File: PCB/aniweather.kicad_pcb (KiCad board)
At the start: 2 copper layers, 55 x 75 mm, 26 parts, among them SW1 SW_DIP_x01, SW2 SW_Push, U5 TPS63001

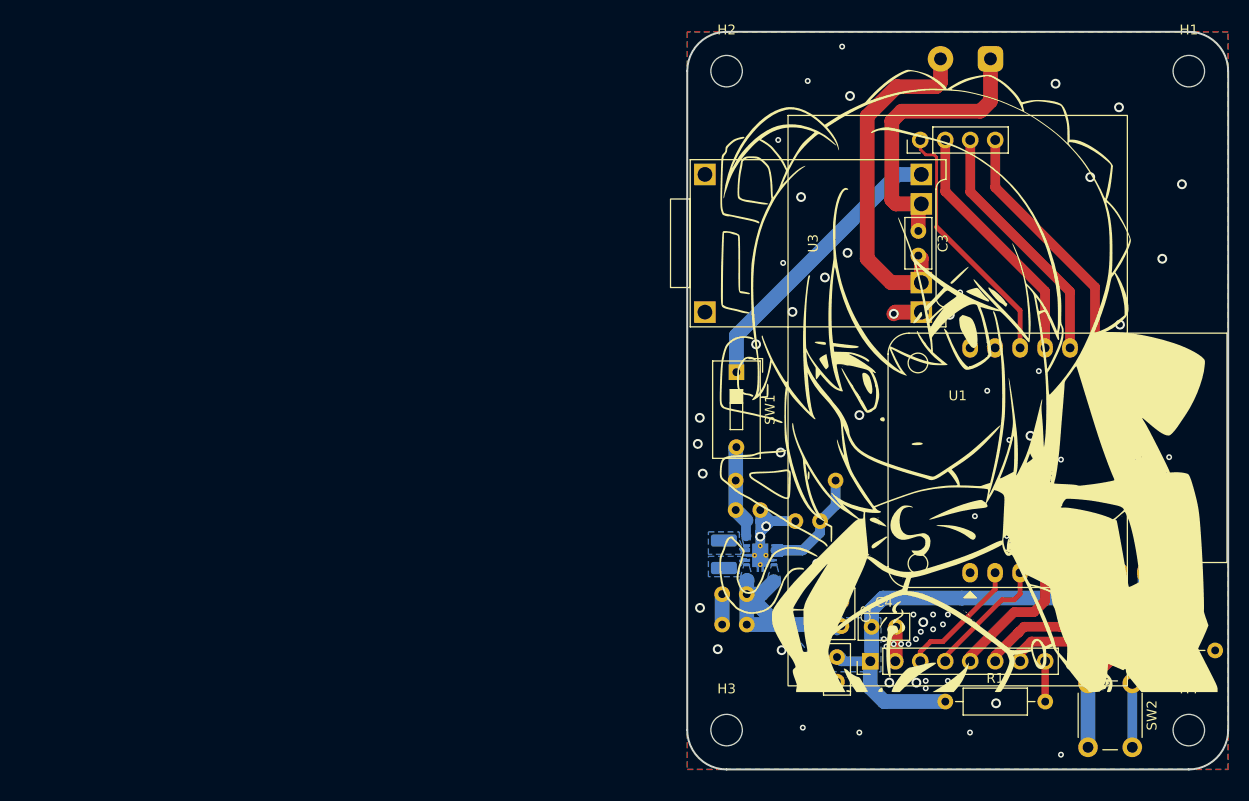
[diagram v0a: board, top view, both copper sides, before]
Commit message: Reroute board
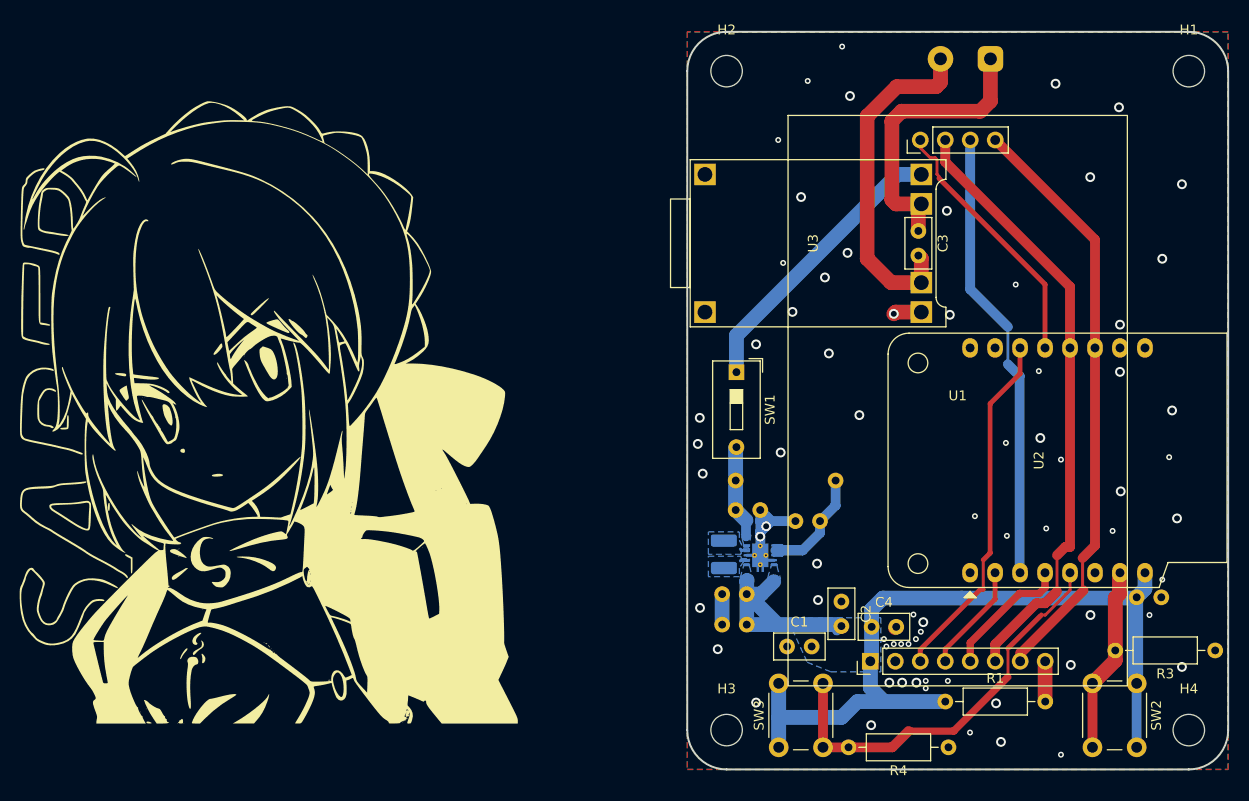
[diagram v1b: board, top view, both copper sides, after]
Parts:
- added R4: 100k, Resistor_THT:R_Axial_DIN0207_L6.3mm_D2.5mm_P10.16mm_Horizontal, F.Cu at (139.3, 136.2)
- added SW3: SW_Push, Button_Switch_THT:SW_PUSH_6mm, F.Cu at (122.0, 136.2)
- moved G1 71.2 mm to (69.2, 98.7)
- moved G2 71.2 mm to (69.2, 98.7)
- moved C1 6.21 mm to (122.8, 125.9), turned to 0 degrees
- moved SW2 0.45 mm to (158.4, 129.7)
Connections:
- U1 pad 10: SD_MISO -> MISO
- U1 pad 11: SD_SCK -> SCK
- U1 pad 5: SDA -> MOSI
- U1 pad 9: SD_MOSI -> MOSI
- U2 pad 0: SDA -> Net-(U2-A0)
- U2 pad 10: SD_CS -> CS_LCD
- U2 pad 2: RESET -> MISO
- U2 pad 3: CS_LCD -> RESET
- U2 pad 4: SCK -> unconnected-(U2-A4-Pad4)
- U2 pad 6: SD_SCK -> SCK
- U2 pad 7: SD_MISO -> MOSI
- U2 pad 8: SD_MOSI -> SD_CS
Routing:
- net MOSI: track 0.00 -> 62.5 mm
- net MISO: track 0.00 -> 46.1 mm
- net SCK: track 15.4 -> 60.4 mm
- net Net-(U2-A0): track 0.00 -> 41.7 mm
- net SD_MISO: track 25.3 -> 0.00 mm
- net SD_SCK: track 25.3 -> 0.00 mm
- net SD_MOSI: track 25.3 -> 0.00 mm
- net CS_LCD: track 12.9 -> 36.2 mm
- net SDA: track 14.7 -> 0.00 mm
- net +3.3V: track 89.2 -> 101.8 mm
- net GND: track 23.3 -> 19.9 mm, vias 72 -> 71
- net RESET: track 12.9 -> 11.1 mm
- net SD_CS: track 25.8 -> 26.7 mm
